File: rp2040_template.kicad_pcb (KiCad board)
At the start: 2 copper layers, 21 x 51 mm, 39 parts, among them J1 USB_C_Receptacle_USB2.0_14P, U1 RP2040, U2 W25Q16JVUXIQ TR, U3 AP2202K-3.3TRG1, Y1 ABM8-272-T3

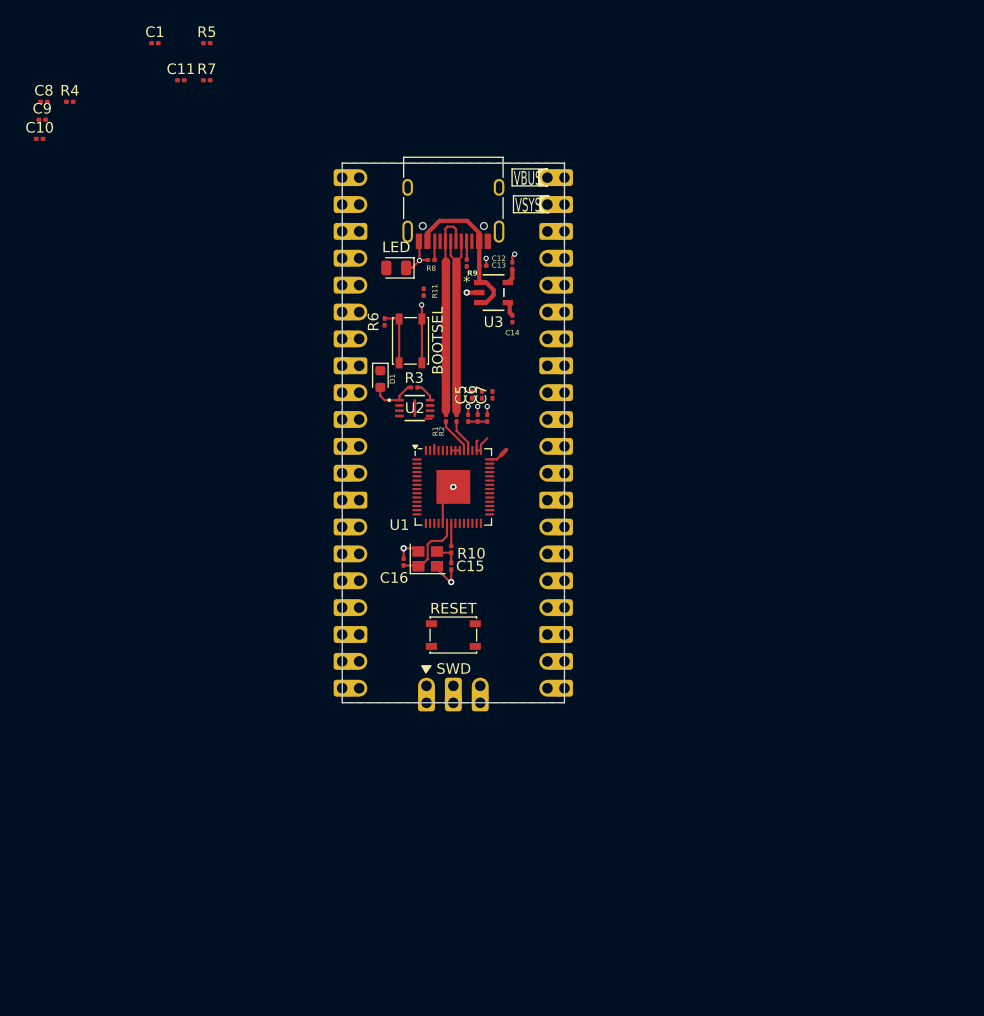
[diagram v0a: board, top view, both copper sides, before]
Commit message: Finished Rev A!
Signed-off-by: Nate <natelostintimeandspace@gmail.com>
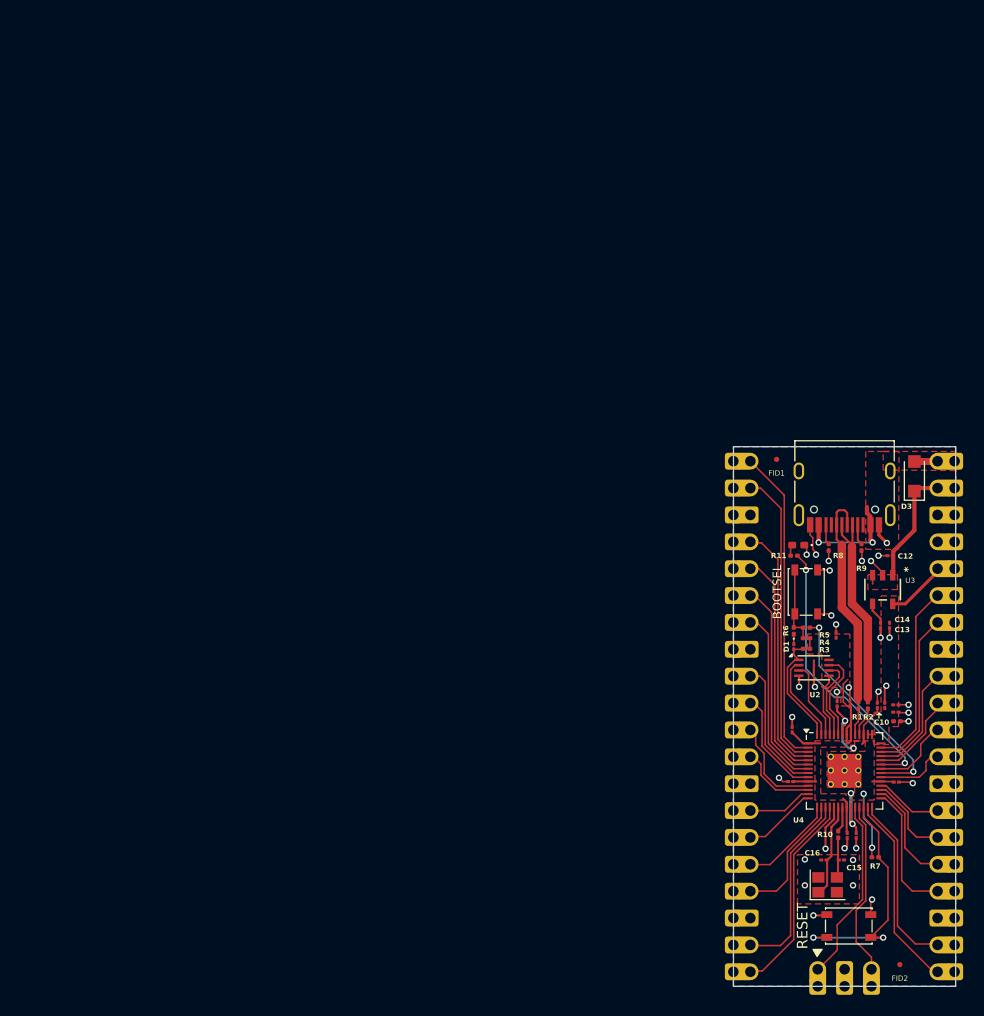
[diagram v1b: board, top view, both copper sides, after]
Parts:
- removed the C2 at (111.9, 74.1)
- removed the REF** at (119.4, 51.4)
- removed the REF** at (101.6, 99.6)
- removed the REF** at (113.0, 99.4)
- removed U1: RP2040, Package_DFN_QFN:QFN-56-1EP_7x7mm_P0.4mm_EP3.2x3.2mm
- added ?: , , F.Cu at (147.5, 107.4)
- added ?: , , F.Cu at (146.2, 107.4)
- added ?: , , F.Cu at (147.5, 108.7)
- added ?: , , F.Cu at (148.8, 107.4)
- added ?: , , F.Cu at (146.2, 108.7)
- added ?: , , F.Cu at (148.8, 108.7)
- added ?: , , F.Cu at (147.5, 106.1)
- added ?: , , F.Cu at (146.2, 106.1)
- added ?: , , F.Cu at (148.8, 106.1)
- added C17: 100nF, Capacitor_SMD:C_01005_0402Metric, F.Cu at (152.4, 108.5)
- added C2: 100nF, Capacitor_SMD:C_0201_0603Metric, F.Cu at (152.4, 102.8)
- added C2: 100nF, Capacitor_SMD:C_01005_0402Metric, F.Cu at (146.7, 94.6)
- added D3: D_Schottky, Diode_SMD:Nexperia_CFP3_SOD-123W, F.Cu at (154.1, 79.6)
- added FID1: Fiducial, Fiducial:Fiducial_0.5mm_Mask1mm, F.Cu at (141.1, 78.0)
- added FID2: Fiducial, Fiducial:Fiducial_0.5mm_Mask1mm, F.Cu at (152.7, 125.8)
- added G***: LOGO, LOGO, B.Cu at (147.1, 120.7)
- added J2: Conn_01x20_Pin, castellated:castellated_tht_1x20, B.Cu at (138.6, 78.2)
- added J3: Conn_01x20_Pin, castellated:castellated_tht_1x20, F.Cu at (156.3, 78.2)
- added J4: Conn_01x03_Pin, castellated:castellated_tht_1x3, F.Cu at (150.0, 126.2)
- added REF**: OSHW-Logo2_7.3x6mm_SilkScreen, Symbol:OSHW-Logo2_7.3x6mm_SilkScreen, B.Cu at (145.7, 90.8)
- added U4: RP2040, Package_DFN_QFN:QFN-56-1EP_7x7mm_P0.4mm_EP3.2x3.2mm, F.Cu at (147.5, 107.4)
- C1, C10, C11, C12, C13, C14, C15, C16, C3, C4, C5, C6, C7, C8, C9: footprint Capacitor_SMD:C_0201_0603Metric -> Capacitor_SMD:C_01005_0402Metric
- D1: footprint Diode_SMD:D_0603_1608Metric -> Diode_SMD:D_01005_0402Metric
- LED1: renamed from LED; footprint LED_SMD:LED_0805_2012Metric -> LED_SMD:LED_0402_1005Metric_Pad0.77x0.64mm_HandSolder
- SW_1: renamed from BOOTSEL; value SW_BOOT -> BOOTSEL
- SW_2: renamed from RESET; value SW_RESET -> RESET
- U2: footprint footprints:USON-8_UX_2x3x0p6_WIN -> Package_SON:Winbond_USON-8-1EP_3x2mm_P0.5mm_EP0.2x1.6mm
- moved R7 96.9 mm to (150.4, 115.6)
- moved C10 95.6 mm to (150.6, 101.2), turned to 90 degrees
- moved C8 95.1 mm to (148.0, 101.1), turned to 90 degrees
- moved C9 94.4 mm to (142.4, 108.5), turned to 180 degrees
- moved C1 94.3 mm to (152.3, 101.9)
- moved C11 89.7 mm to (152.3, 101.2)
- moved R4 86.1 mm to (143.9, 94.9), turned to 180 degrees
- moved R5 79.1 mm to (143.9, 93.9)
- moved C5 54.7 mm to (147.7, 113.5), turned to -90 degrees
- moved C6 54.6 mm to (148.6, 113.5), turned to -90 degrees
- moved C13 49.3 mm to (151.7, 93.7), turned to -90 degrees
- moved Y1 48.8 mm to (145.9, 118.2)
- moved C16 48.7 mm to (145.5, 115.9), turned to 0 degrees
- moved R6 48.5 mm to (142.7, 94.2)
- moved R1 47.5 mm to (148.8, 101.2)
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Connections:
- C10 pad 1: Net-(U1-VREG_VOUT) -> +1V1
- C12 pad 1: VBUS -> /VSYS
- C6 pad 1: +3V3 -> +1V1
- C7 pad 1: +3V3 -> +1V1
- C8 pad 1: Net-(U1-VREG_VOUT) -> +3V3
- C9 pad 1: Net-(U1-VREG_VOUT) -> +3V3
- U3 pad 1: VBUS -> /VSYS
- U3 pad 3: VBUS -> /VSYS
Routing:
- net /GPIO0: track 0.00 -> 30.1 mm
- net /GPIO1: track 0.00 -> 28.5 mm
- net /USER_LED: track 0.00 -> 26.7 mm, vias 0 -> 2
- net /GPIO2: track 0.00 -> 23.8 mm
- net /RESET: track 0.00 -> 23.0 mm, vias 0 -> 2
- net +3V3: track 10.7 -> 33.2 mm, vias 0 -> 2
- net /GPIO3: track 0.00 -> 21.6 mm
- net /USER_SW: track 0.00 -> 21.3 mm, vias 0 -> 2
- net /GPIO15: track 0.00 -> 19.3 mm
- net /GPIO4: track 0.00 -> 19.3 mm
- net /GPIO16: track 0.00 -> 18.5 mm
- net /GPIO14: track 0.00 -> 17.7 mm
- net /ADC3: track 0.00 -> 17.6 mm
- net /SWCLK: track 0.00 -> 17.4 mm
- net /GPIO5: track 0.00 -> 17.3 mm
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- added copper zone on F.Cu, net +1V1
- added copper zone on F.Cu, net +3V3
- added copper zone on F.Cu, net /VSYS
- added copper zone on F.Cu, net GND
- added copper zone on F.Cu, net VBUS
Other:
- rule pad_to_mask_clearance: 0 -> 0.051
- board text added: "+3V3"
- board text added: "A0"
- board text added: "A1"
- board text added: "A2"
- board text added: "A3"
- board text added: "CLK"
- board text added: "DIO"
- board text added: "GND"
- board text added: "GP0"
- board text added: "GP1"
- board text added: "GP10"
- board text added: "GP11"
- board text added: "GP12"
- board text added: "GP13"
- board text added: "GP14"
- board text added: "GP15"
- board text added: "GP16"
- board text added: "GP17"
- board text added: "GP18"
- board text added: "GP19"
- board text added: "GP2"
- board text added: "GP20"
- board text added: "GP21"
- board text added: "GP22"
- board text added: "GP24"
- board text added: "GP3"
- board text added: "GP4"
- board text added: "GP5"
- board text added: "GP6"
- board text added: "GP7"
- board text added: "GP8"
- board text added: "GP9"
- board text added: "N.W. 2024 Rev A"
- board text added: "NC"
- board text added: "RP2040"
